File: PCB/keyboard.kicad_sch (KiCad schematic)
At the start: 139 parts, among them SW1 SW_Push, SW10 SW_Push, SW11 SW_Push, SW12 SW_Push, SW13 SW_Push, SW14 SW_Push, SW15 SW_Push, SW16 SW_Push, SW17 SW_Push, SW18 SW_Push, SW19 SW_Push, SW2 SW_Push, SW20 SW_Push, SW21 SW_Push, SW22 SW_Push, SW23 SW_Push, SW24 SW_Push, SW25 SW_Push, SW26 SW_Push, SW27 SW_Push, SW28 SW_Push, SW29 SW_Push, SW3 SW_Push, SW30 SW_Push, SW31 SW_Push, SW32 SW_Push, SW33 SW_Push, SW34 SW_Push, SW35 SW_Push, SW36 SW_Push, SW37 SW_Push, SW38 SW_Push, SW39 SW_Push, SW4 SW_Push, SW40 SW_Push, SW41 SW_Push, SW42 SW_Push, SW43 SW_Push, SW44 SW_Push, SW45 SW_Push, SW46 SW_Push, SW47 SW_Push, SW48 SW_Push, SW49 SW_Push, SW5 SW_Push, SW50 SW_Push, SW51 SW_Push, SW52 SW_Push, SW53 SW_Push, SW54 SW_Push, SW55 SW_Push, SW56 SW_Push, SW57 SW_Push, SW58 SW_Push, SW59 SW_Push, SW6 SW_Push, SW60 SW_Push, SW61 SW_Push, SW62 RotaryEncoder_Switch, SW63 RotaryEncoder_Switch, SW7 SW_Push, SW8 SW_Push, SW9 SW_Push, U1 Pico

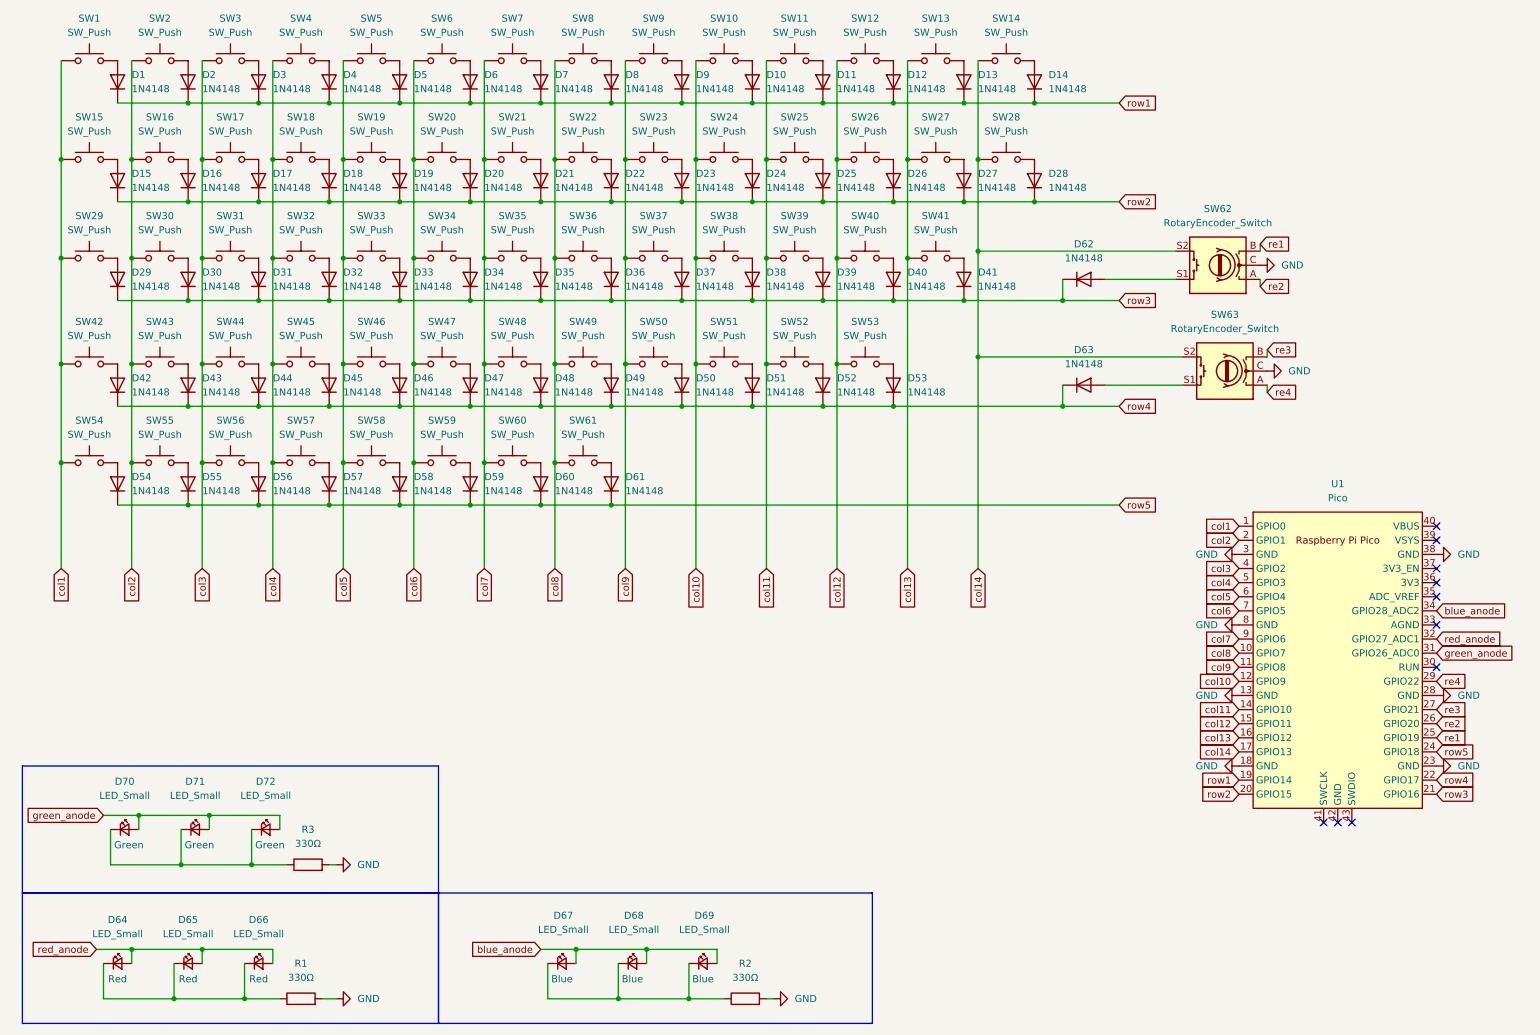
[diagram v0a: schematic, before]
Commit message: updated PCB
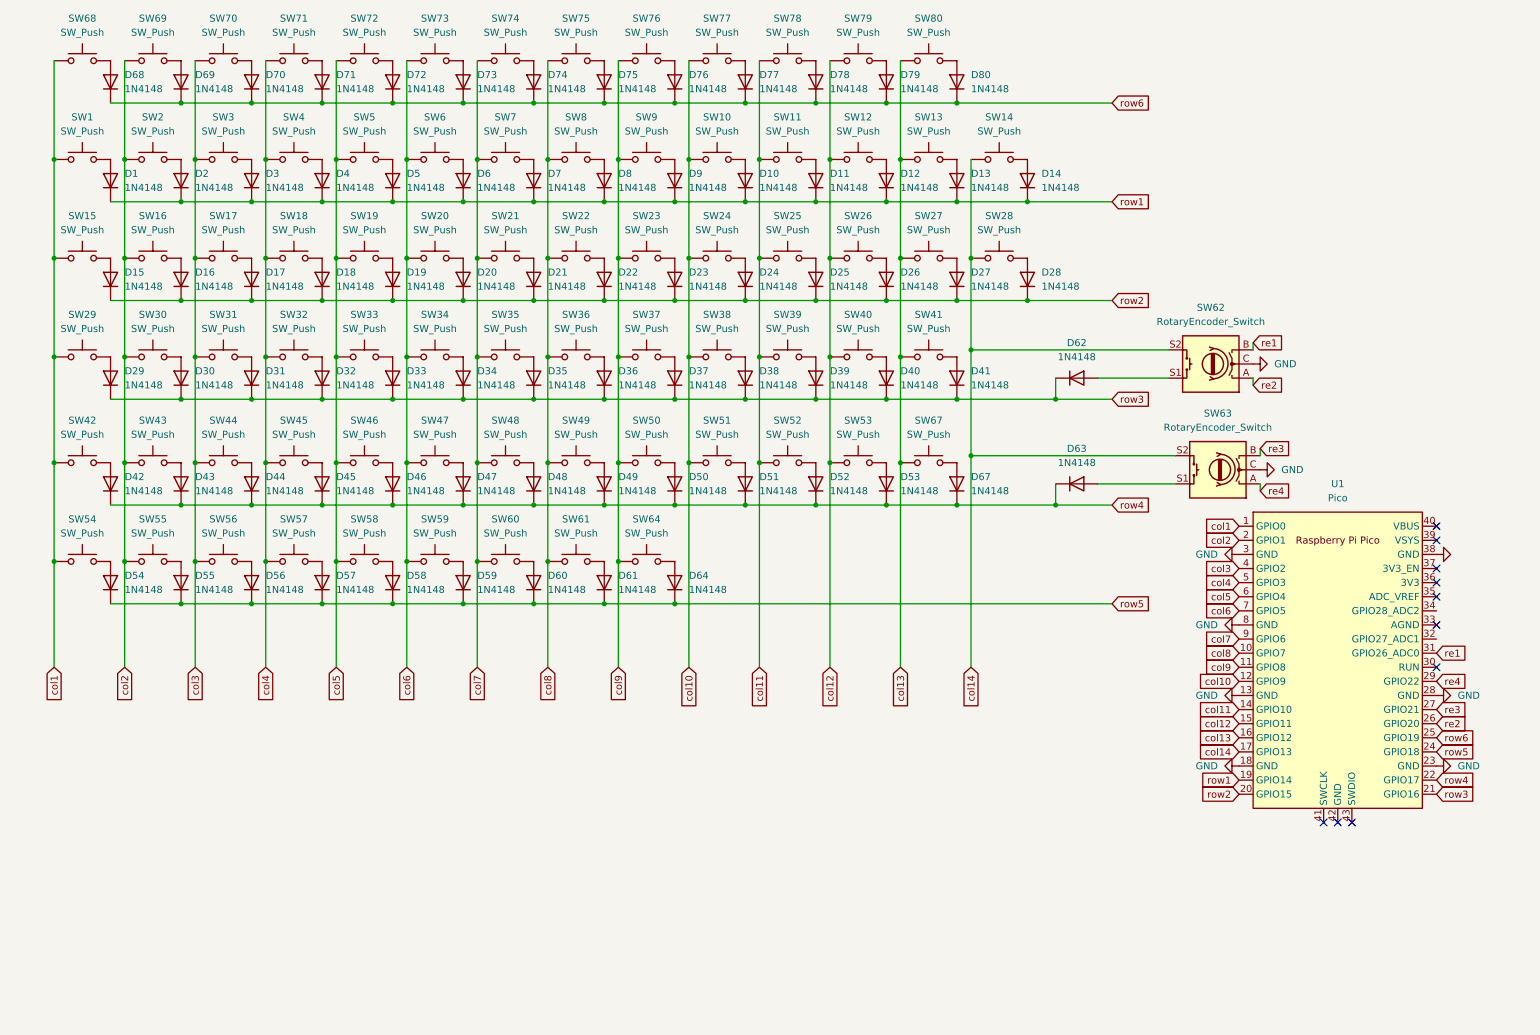
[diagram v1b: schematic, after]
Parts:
- removed D64, D65, D66, D67, D68, D69, D70, D71, D72: LED_Small, LED_THT:LED_D5.0mm, symbol Device:LED_Small
- removed R1, R2, R3: 330Ω, Resistor_THT:R_Axial_DIN0309_L9.0mm_D3.2mm_P20.32mm_Horizontal, symbol Device:R
- added D64, D67, D68, D69, D70, D71, D72, D73, D74, D75, D76, D77, D78, D79, D80: 1N4148, Diode_THT:D_DO-35_SOD27_P7.62mm_Horizontal, symbol Diode:1N4148
- added SW64, SW67, SW68, SW69, SW70, SW71, SW72, SW73, SW74, SW75, SW76, SW77, SW78, SW79, SW80: SW_Push, Button_Switch_Keyboard:SW_Cherry_MX_1.00u_PCB, symbol Switch:SW_Push
- SW53: footprint Button_Switch_Keyboard:SW_Cherry_MX_2.75u_PCB -> Button_Switch_Keyboard:SW_Cherry_MX_1.75u_PCB
- SW60, SW61: footprint Button_Switch_Keyboard:SW_Cherry_MX_1.25u_PCB -> Button_Switch_Keyboard:SW_Cherry_MX_1.00u_PCB
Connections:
- net green_anode is gone; now on net re1: U1.31 (GPIO26_ADC0)
- net col1: now also SW68.1
- net col10: now also SW77.1
- net col11: now also SW78.1
- net col12: now also SW79.1
- net col13: now also SW67.1, SW80.1
- net col2: now also SW69.1
- net col3: now also SW70.1
- net col4: now also SW71.1
- net col5: now also SW72.1
- net col6: now also SW73.1
- net col7: now also SW74.1
- net col8: now also SW75.1
- net col9: now also SW64.1, SW76.1
- net re1: no longer U1.25 (GPIO19)
- net row4: now also D67.1 (K)
- net row5: now also D64.1 (K)
- net blue_anode: no longer names the net of U1.34 (GPIO28_ADC2)
- net red_anode: no longer names the net of U1.32 (GPIO27_ADC1)
- new net: D72.2 (A), SW72.2
- new net: D76.2 (A), SW76.2
- new net: D78.2 (A), SW78.2
- new net: D64.2 (A), SW64.2
- new net: D73.2 (A), SW73.2
- new net: D69.2 (A), SW69.2
- new net: D75.2 (A), SW75.2
- new net: D70.2 (A), SW70.2
- new net: D71.2 (A), SW71.2
- new net: D74.2 (A), SW74.2
- new net: D77.2 (A), SW77.2
- new net: D79.2 (A), SW79.2
- new net: D80.2 (A), SW80.2
- new net: D67.2 (A), SW67.2
- new net: D68.2 (A), SW68.2
- new net row6: D68.1 (K), D69.1 (K), D70.1 (K), D71.1 (K), D72.1 (K), D73.1 (K), D74.1 (K), D75.1 (K), D76.1 (K), D77.1 (K), D78.1 (K), D79.1 (K), D80.1 (K), U1.25 (GPIO19)
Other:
- moved on the sheet: D1, D10, D11, D12, D13, D14, D15, D16, D17, D18, D19, D2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
